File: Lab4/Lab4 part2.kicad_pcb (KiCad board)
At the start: 2 copper layers, 58.4 x 50.4 mm, 10 parts, among them J1 Conn_01x02_Male, U1 NE555D

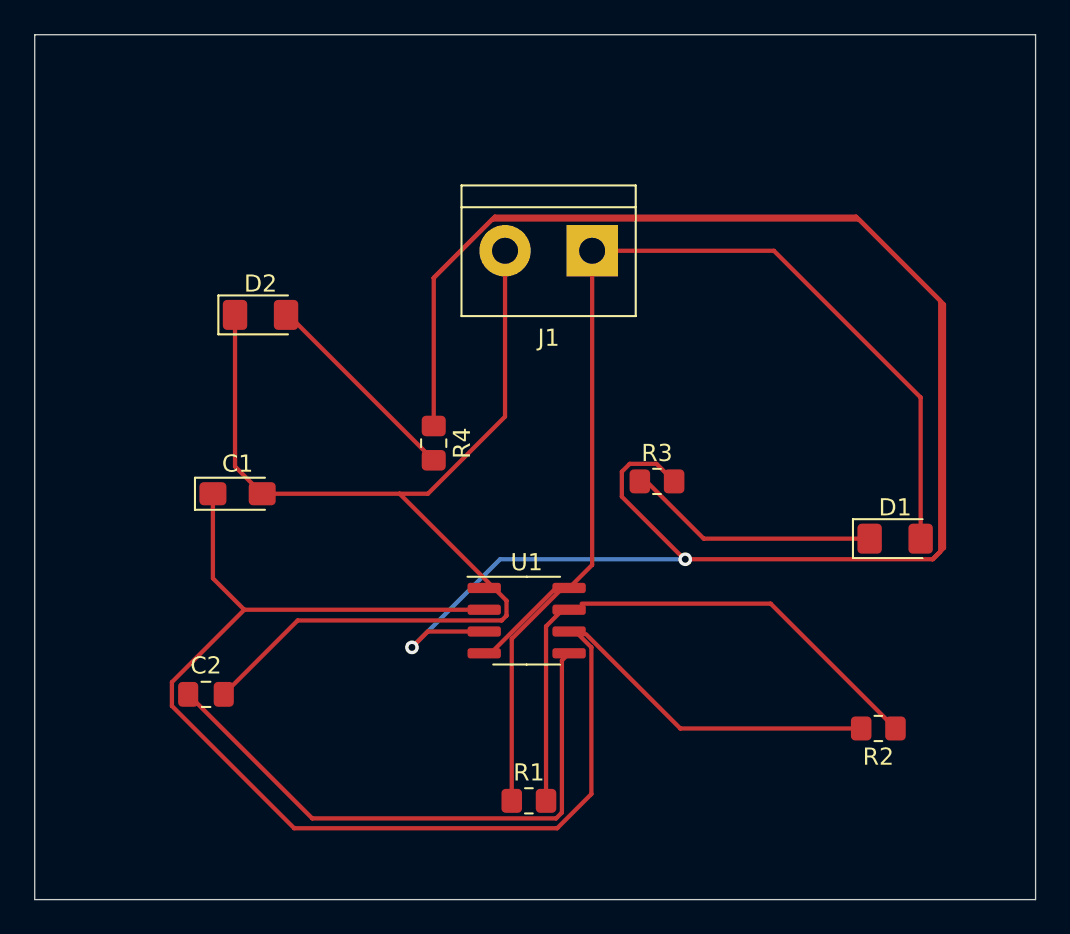
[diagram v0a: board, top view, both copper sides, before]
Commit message: update lab7
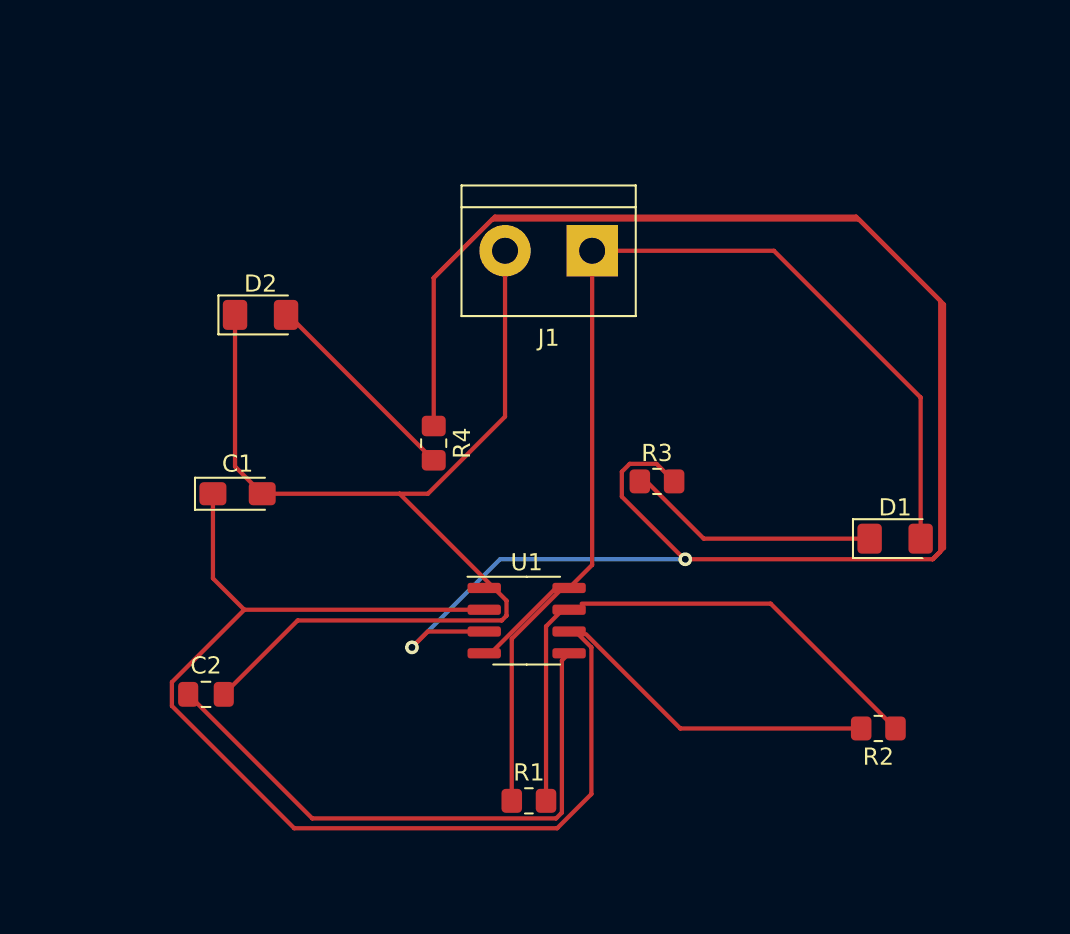
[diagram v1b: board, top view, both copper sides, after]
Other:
- board outline removed
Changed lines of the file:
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@@
       (outputformat 1)
       (mirror false)
-      (drillshape 0)
+      (drillshape 1)
       (scaleselection 1)
-      (outputdirectory "lab7/")
+      (outputdirectory "")
     )
   )
@@
     (fp_line (start 1.6 0.8) (end 1.6 -0.8) (layer "F.Fab") (width 0.1))
     (fp_line (start -1.2 -0.8) (end -1.6 -0.4) (layer "F.Fab") (width 0.1))
-    (pad "1" smd roundrect (at -1.4875 0) (size 1.425 1.75) (layers "F.Cu" "F.Paste" "F.Mask") (roundrect_rratio 0.1754392982)
+    (pad "1" smd roundrect (at -1.4875 0) (size 1.425 1.75) (layers "F.Cu" "F.Paste" "F.Mask") (roundrect_rratio 0.175439)
       (net 4 "Net-(D1-Pad1)") (pinfunction "K") (pintype "passive"))
-    (pad "2" smd roundrect (at 1.4875 0) (size 1.425 1.75) (layers "F.Cu" "F.Paste" "F.Mask") (roundrect_rratio 0.1754392982)
+    (pad "2" smd roundrect (at 1.4875 0) (size 1.425 1.75) (layers "F.Cu" "F.Paste" "F.Mask") (roundrect_rratio 0.175439)
       (net 5 "+9V") (pinfunction "A") (pintype "passive"))
     (model "${KICAD6_3DMODEL_DIR}/LED_SMD.3dshapes/LED_1206_3216Metric.wrl"
@@
     (fp_line (start 1.6 0.8) (end 1.6 -0.8) (layer "F.Fab") (width 0.1))
     (fp_line (start 1.6 -0.8) (end -1.2 -0.8) (layer "F.Fab") (width 0.1))
-    (pad "1" smd roundrect (at -1.4375 0) (size 1.575 1.35) (layers "F.Cu" "F.Paste" "F.Mask") (roundrect_rratio 0.1851851852)
+    (pad "1" smd roundrect (at -1.4375 0) (size 1.575 1.35) (layers "F.Cu" "F.Paste" "F.Mask") (roundrect_rratio 0.185185)
       (net 1 "/pin_2") (pintype "passive"))
-    (pad "2" smd roundrect (at 1.4375 0) (size 1.575 1.35) (layers "F.Cu" "F.Paste" "F.Mask") (roundrect_rratio 0.1851851852)
+    (pad "2" smd roundrect (at 1.4375 0) (size 1.575 1.35) (layers "F.Cu" "F.Paste" "F.Mask") (roundrect_rratio 0.185185)
       (net 2 "GND") (pintype "passive"))
     (model "${KICAD6_3DMODEL_DIR}/Capacitor_Tantalum_SMD.3dshapes/CP_EIA-3216-18_Kemet-A.wrl"
@@
     (fp_line (start -1 0.625) (end -1 -0.625) (layer "F.Fab") (width 0.1))
     (fp_line (start 1 -0.625) (end 1 0.625) (layer "F.Fab") (width 0.1))
-    (pad "1" smd roundrect (at -1 0 180) (size 1.2 1.4) (layers "F.Cu" "F.Paste" "F.Mask") (roundrect_rratio 0.2083333333)
+    (pad "1" smd roundrect (at -1 0 180) (size 1.2 1.4) (layers "F.Cu" "F.Paste" "F.Mask") (roundrect_rratio 0.208333)
       (net 7 "/pin_7") (pintype "passive"))
-    (pad "2" smd roundrect (at 1 0 180) (size 1.2 1.4) (layers "F.Cu" "F.Paste" "F.Mask") (roundrect_rratio 0.2083333333)
+    (pad "2" smd roundrect (at 1 0 180) (size 1.2 1.4) (layers "F.Cu" "F.Paste" "F.Mask") (roundrect_rratio 0.208333)
       (net 1 "/pin_2") (pintype "passive"))
     (model "${KICAD6_3DMODEL_DIR}/Resistor_SMD.3dshapes/R_0805_2012Metric.wrl"
@@
     (fp_line (start -1 0.625) (end -1 -0.625) (layer "F.Fab") (width 0.1))
     (fp_line (start -1 -0.625) (end 1 -0.625) (layer "F.Fab") (width 0.1))
-    (pad "1" smd roundrect (at -1 0) (size 1.2 1.4) (layers "F.Cu" "F.Paste" "F.Mask") (roundrect_rratio 0.2083333333)
+    (pad "1" smd roundrect (at -1 0) (size 1.2 1.4) (layers "F.Cu" "F.Paste" "F.Mask") (roundrect_rratio 0.208333)
       (net 5 "+9V") (pintype "passive"))
-    (pad "2" smd roundrect (at 1 0) (size 1.2 1.4) (layers "F.Cu" "F.Paste" "F.Mask") (roundrect_rratio 0.2083333333)
+    (pad "2" smd roundrect (at 1 0) (size 1.2 1.4) (layers "F.Cu" "F.Paste" "F.Mask") (roundrect_rratio 0.208333)
       (net 7 "/pin_7") (pintype "passive"))
     (model "${KICAD6_3DMODEL_DIR}/Resistor_SMD.3dshapes/R_0805_2012Metric.wrl"
@@
     (fp_line (start -1 0.625) (end -1 -0.625) (layer "F.Fab") (width 0.1))
     (fp_line (start 1 -0.625) (end 1 0.625) (layer "F.Fab") (width 0.1))
-    (pad "1" smd roundrect (at -1 0 270) (size 1.2 1.4) (layers "F.Cu" "F.Paste" "F.Mask") (roundrect_rratio 0.2083333333)
+    (pad "1" smd roundrect (at -1 0 270) (size 1.2 1.4) (layers "F.Cu" "F.Paste" "F.Mask") (roundrect_rratio 0.208333)
       (net 8 "/pin_3") (pintype "passive"))
-    (pad "2" smd roundrect (at 1 0 270) (size 1.2 1.4) (layers "F.Cu" "F.Paste" "F.Mask") (roundrect_rratio 0.2083333333)
+    (pad "2" smd roundrect (at 1 0 270) (size 1.2 1.4) (layers "F.Cu" "F.Paste" "F.Mask") (roundrect_rratio 0.208333)
       (net 6 "Net-(D2-Pad2)") (pintype "passive"))
     (model "${KICAD6_3DMODEL_DIR}/Resistor_SMD.3dshapes/R_0805_2012Metric.wrl"
@@
     (fp_line (start 1 0.625) (end -1 0.625) (layer "F.Fab") (width 0.1))
     (fp_line (start 1 -0.625) (end 1 0.625) (layer "F.Fab") (width 0.1))
-    (pad "1" smd roundrect (at -1.0375 0) (size 1.175 1.45) (layers "F.Cu" "F.Paste" "F.Mask") (roundrect_rratio 0.2127659574)
+    (pad "1" smd roundrect (at -1.0375 0) (size 1.175 1.45) (layers "F.Cu" "F.Paste" "F.Mask") (roundrect_rratio 0.212766)
       (net 3 "Net-(C2-Pad1)") (pintype "passive"))
-    (pad "2" smd roundrect (at 1.0375 0) (size 1.175 1.45) (layers "F.Cu" "F.Paste" "F.Mask") (roundrect_rratio 0.2127659574)
+    (pad "2" smd roundrect (at 1.0375 0) (size 1.175 1.45) (layers "F.Cu" "F.Paste" "F.Mask") (roundrect_rratio 0.212766)
       (net 2 "GND") (pintype "passive"))
     (model "${KICAD6_3DMODEL_DIR}/Capacitor_SMD.3dshapes/C_0805_2012Metric.wrl"
@@
     (fp_line (start 1 0.625) (end -1 0.625) (layer "F.Fab") (width 0.1))
     (fp_line (start 1 -0.625) (end 1 0.625) (layer "F.Fab") (width 0.1))
-    (pad "1" smd roundrect (at -1 0) (size 1.2 1.4) (layers "F.Cu" "F.Paste" "F.Mask") (roundrect_rratio 0.2083333333)
+    (pad "1" smd roundrect (at -1 0) (size 1.2 1.4) (layers "F.Cu" "F.Paste" "F.Mask") (roundrect_rratio 0.208333)
       (net 4 "Net-(D1-Pad1)") (pintype "passive"))
-    (pad "2" smd roundrect (at 1 0) (size 1.2 1.4) (layers "F.Cu" "F.Paste" "F.Mask") (roundrect_rratio 0.2083333333)
+    (pad "2" smd roundrect (at 1 0) (size 1.2 1.4) (layers "F.Cu" "F.Paste" "F.Mask") (roundrect_rratio 0.208333)
       (net 8 "/pin_3") (pintype "passive"))
     (model "${KICAD6_3DMODEL_DIR}/Resistor_SMD.3dshapes/R_0805_2012Metric.wrl"
@@
     (fp_line (start 1.6 -0.8) (end -1.2 -0.8) (layer "F.Fab") (width 0.1))
     (fp_line (start -1.2 -0.8) (end -1.6 -0.4) (layer "F.Fab") (width 0.1))
-    (pad "1" smd roundrect (at -1.4875 0) (size 1.425 1.75) (layers "F.Cu" "F.Paste" "F.Mask") (roundrect_rratio 0.1754392982)
+    (pad "1" smd roundrect (at -1.4875 0) (size 1.425 1.75) (layers "F.Cu" "F.Paste" "F.Mask") (roundrect_rratio 0.175439)
       (net 2 "GND") (pinfunction "K") (pintype "passive"))
-    (pad "2" smd roundrect (at 1.4875 0) (size 1.425 1.75) (layers "F.Cu" "F.Paste" "F.Mask") (roundrect_rratio 0.1754392982)
+    (pad "2" smd roundrect (at 1.4875 0) (size 1.425 1.75) (layers "F.Cu" "F.Paste" "F.Mask") (roundrect_rratio 0.175439)
       (net 6 "Net-(D2-Pad2)") (pinfunction "A") (pintype "passive"))
     (model "${KICAD6_3DMODEL_DIR}/LED_SMD.3dshapes/LED_1206_3216Metric.wrl"
@@
     )
   )
-  (gr_rect (start 110.83 57.61) (end 169.2 108.05) (layer "Edge.Cuts") (width 0.05) (fill none))
   (segment (start 121.2225 84.38) (end 121.2225 89.3125) (width 0.25) (layer "F.Cu") (net 1))
   (segment (start 123.055 91.145) (end 137.045 91.145) (width 0.25) (layer "F.Cu") (net 1))

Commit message: my lab8 update, tks
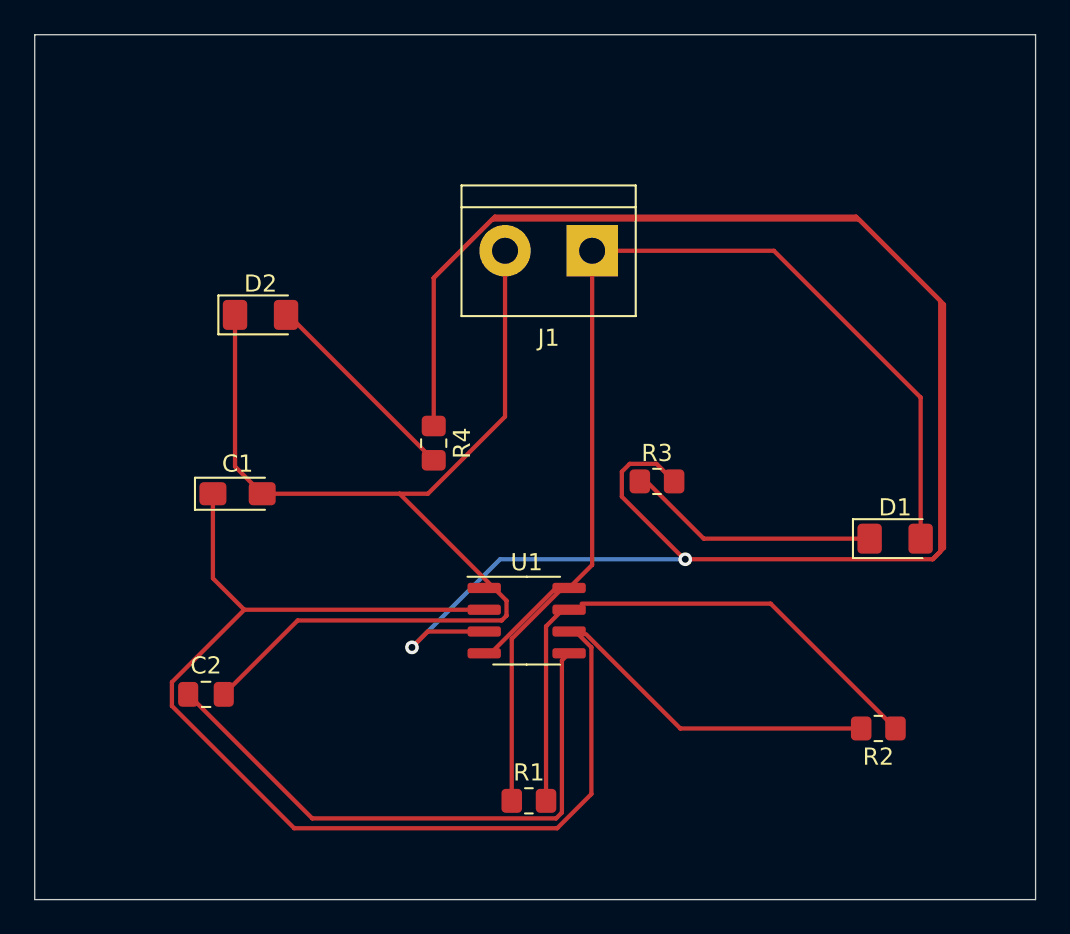
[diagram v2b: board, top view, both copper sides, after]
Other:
- board outline added: 58.4 x 50.4 mm
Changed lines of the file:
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@@
       (outputformat 1)
       (mirror false)
-      (drillshape 1)
+      (drillshape 0)
       (scaleselection 1)
-      (outputdirectory "")
+      (outputdirectory "lab7/")
     )
   )
@@
     (fp_line (start 1.6 0.8) (end 1.6 -0.8) (layer "F.Fab") (width 0.1))
     (fp_line (start -1.2 -0.8) (end -1.6 -0.4) (layer "F.Fab") (width 0.1))
-    (pad "1" smd roundrect (at -1.4875 0) (size 1.425 1.75) (layers "F.Cu" "F.Paste" "F.Mask") (roundrect_rratio 0.175439)
+    (pad "1" smd roundrect (at -1.4875 0) (size 1.425 1.75) (layers "F.Cu" "F.Paste" "F.Mask") (roundrect_rratio 0.1754392982)
       (net 4 "Net-(D1-Pad1)") (pinfunction "K") (pintype "passive"))
-    (pad "2" smd roundrect (at 1.4875 0) (size 1.425 1.75) (layers "F.Cu" "F.Paste" "F.Mask") (roundrect_rratio 0.175439)
+    (pad "2" smd roundrect (at 1.4875 0) (size 1.425 1.75) (layers "F.Cu" "F.Paste" "F.Mask") (roundrect_rratio 0.1754392982)
       (net 5 "+9V") (pinfunction "A") (pintype "passive"))
     (model "${KICAD6_3DMODEL_DIR}/LED_SMD.3dshapes/LED_1206_3216Metric.wrl"
@@
     (fp_line (start 1.6 0.8) (end 1.6 -0.8) (layer "F.Fab") (width 0.1))
     (fp_line (start 1.6 -0.8) (end -1.2 -0.8) (layer "F.Fab") (width 0.1))
-    (pad "1" smd roundrect (at -1.4375 0) (size 1.575 1.35) (layers "F.Cu" "F.Paste" "F.Mask") (roundrect_rratio 0.185185)
+    (pad "1" smd roundrect (at -1.4375 0) (size 1.575 1.35) (layers "F.Cu" "F.Paste" "F.Mask") (roundrect_rratio 0.1851851852)
       (net 1 "/pin_2") (pintype "passive"))
-    (pad "2" smd roundrect (at 1.4375 0) (size 1.575 1.35) (layers "F.Cu" "F.Paste" "F.Mask") (roundrect_rratio 0.185185)
+    (pad "2" smd roundrect (at 1.4375 0) (size 1.575 1.35) (layers "F.Cu" "F.Paste" "F.Mask") (roundrect_rratio 0.1851851852)
       (net 2 "GND") (pintype "passive"))
     (model "${KICAD6_3DMODEL_DIR}/Capacitor_Tantalum_SMD.3dshapes/CP_EIA-3216-18_Kemet-A.wrl"
@@
     (fp_line (start -1 0.625) (end -1 -0.625) (layer "F.Fab") (width 0.1))
     (fp_line (start 1 -0.625) (end 1 0.625) (layer "F.Fab") (width 0.1))
-    (pad "1" smd roundrect (at -1 0 180) (size 1.2 1.4) (layers "F.Cu" "F.Paste" "F.Mask") (roundrect_rratio 0.208333)
+    (pad "1" smd roundrect (at -1 0 180) (size 1.2 1.4) (layers "F.Cu" "F.Paste" "F.Mask") (roundrect_rratio 0.2083333333)
       (net 7 "/pin_7") (pintype "passive"))
-    (pad "2" smd roundrect (at 1 0 180) (size 1.2 1.4) (layers "F.Cu" "F.Paste" "F.Mask") (roundrect_rratio 0.208333)
+    (pad "2" smd roundrect (at 1 0 180) (size 1.2 1.4) (layers "F.Cu" "F.Paste" "F.Mask") (roundrect_rratio 0.2083333333)
       (net 1 "/pin_2") (pintype "passive"))
     (model "${KICAD6_3DMODEL_DIR}/Resistor_SMD.3dshapes/R_0805_2012Metric.wrl"
@@
     (fp_line (start -1 0.625) (end -1 -0.625) (layer "F.Fab") (width 0.1))
     (fp_line (start -1 -0.625) (end 1 -0.625) (layer "F.Fab") (width 0.1))
-    (pad "1" smd roundrect (at -1 0) (size 1.2 1.4) (layers "F.Cu" "F.Paste" "F.Mask") (roundrect_rratio 0.208333)
+    (pad "1" smd roundrect (at -1 0) (size 1.2 1.4) (layers "F.Cu" "F.Paste" "F.Mask") (roundrect_rratio 0.2083333333)
       (net 5 "+9V") (pintype "passive"))
-    (pad "2" smd roundrect (at 1 0) (size 1.2 1.4) (layers "F.Cu" "F.Paste" "F.Mask") (roundrect_rratio 0.208333)
+    (pad "2" smd roundrect (at 1 0) (size 1.2 1.4) (layers "F.Cu" "F.Paste" "F.Mask") (roundrect_rratio 0.2083333333)
       (net 7 "/pin_7") (pintype "passive"))
     (model "${KICAD6_3DMODEL_DIR}/Resistor_SMD.3dshapes/R_0805_2012Metric.wrl"
@@
     (fp_line (start -1 0.625) (end -1 -0.625) (layer "F.Fab") (width 0.1))
     (fp_line (start 1 -0.625) (end 1 0.625) (layer "F.Fab") (width 0.1))
-    (pad "1" smd roundrect (at -1 0 270) (size 1.2 1.4) (layers "F.Cu" "F.Paste" "F.Mask") (roundrect_rratio 0.208333)
+    (pad "1" smd roundrect (at -1 0 270) (size 1.2 1.4) (layers "F.Cu" "F.Paste" "F.Mask") (roundrect_rratio 0.2083333333)
       (net 8 "/pin_3") (pintype "passive"))
-    (pad "2" smd roundrect (at 1 0 270) (size 1.2 1.4) (layers "F.Cu" "F.Paste" "F.Mask") (roundrect_rratio 0.208333)
+    (pad "2" smd roundrect (at 1 0 270) (size 1.2 1.4) (layers "F.Cu" "F.Paste" "F.Mask") (roundrect_rratio 0.2083333333)
       (net 6 "Net-(D2-Pad2)") (pintype "passive"))
     (model "${KICAD6_3DMODEL_DIR}/Resistor_SMD.3dshapes/R_0805_2012Metric.wrl"
@@
     (fp_line (start 1 0.625) (end -1 0.625) (layer "F.Fab") (width 0.1))
     (fp_line (start 1 -0.625) (end 1 0.625) (layer "F.Fab") (width 0.1))
-    (pad "1" smd roundrect (at -1.0375 0) (size 1.175 1.45) (layers "F.Cu" "F.Paste" "F.Mask") (roundrect_rratio 0.212766)
+    (pad "1" smd roundrect (at -1.0375 0) (size 1.175 1.45) (layers "F.Cu" "F.Paste" "F.Mask") (roundrect_rratio 0.2127659574)
       (net 3 "Net-(C2-Pad1)") (pintype "passive"))
-    (pad "2" smd roundrect (at 1.0375 0) (size 1.175 1.45) (layers "F.Cu" "F.Paste" "F.Mask") (roundrect_rratio 0.212766)
+    (pad "2" smd roundrect (at 1.0375 0) (size 1.175 1.45) (layers "F.Cu" "F.Paste" "F.Mask") (roundrect_rratio 0.2127659574)
       (net 2 "GND") (pintype "passive"))
     (model "${KICAD6_3DMODEL_DIR}/Capacitor_SMD.3dshapes/C_0805_2012Metric.wrl"
@@
     (fp_line (start 1 0.625) (end -1 0.625) (layer "F.Fab") (width 0.1))
     (fp_line (start 1 -0.625) (end 1 0.625) (layer "F.Fab") (width 0.1))
-    (pad "1" smd roundrect (at -1 0) (size 1.2 1.4) (layers "F.Cu" "F.Paste" "F.Mask") (roundrect_rratio 0.208333)
+    (pad "1" smd roundrect (at -1 0) (size 1.2 1.4) (layers "F.Cu" "F.Paste" "F.Mask") (roundrect_rratio 0.2083333333)
       (net 4 "Net-(D1-Pad1)") (pintype "passive"))
-    (pad "2" smd roundrect (at 1 0) (size 1.2 1.4) (layers "F.Cu" "F.Paste" "F.Mask") (roundrect_rratio 0.208333)
+    (pad "2" smd roundrect (at 1 0) (size 1.2 1.4) (layers "F.Cu" "F.Paste" "F.Mask") (roundrect_rratio 0.2083333333)
       (net 8 "/pin_3") (pintype "passive"))
     (model "${KICAD6_3DMODEL_DIR}/Resistor_SMD.3dshapes/R_0805_2012Metric.wrl"
@@
     (fp_line (start 1.6 -0.8) (end -1.2 -0.8) (layer "F.Fab") (width 0.1))
     (fp_line (start -1.2 -0.8) (end -1.6 -0.4) (layer "F.Fab") (width 0.1))
-    (pad "1" smd roundrect (at -1.4875 0) (size 1.425 1.75) (layers "F.Cu" "F.Paste" "F.Mask") (roundrect_rratio 0.175439)
+    (pad "1" smd roundrect (at -1.4875 0) (size 1.425 1.75) (layers "F.Cu" "F.Paste" "F.Mask") (roundrect_rratio 0.1754392982)
       (net 2 "GND") (pinfunction "K") (pintype "passive"))
-    (pad "2" smd roundrect (at 1.4875 0) (size 1.425 1.75) (layers "F.Cu" "F.Paste" "F.Mask") (roundrect_rratio 0.175439)
+    (pad "2" smd roundrect (at 1.4875 0) (size 1.425 1.75) (layers "F.Cu" "F.Paste" "F.Mask") (roundrect_rratio 0.1754392982)
       (net 6 "Net-(D2-Pad2)") (pinfunction "A") (pintype "passive"))
     (model "${KICAD6_3DMODEL_DIR}/LED_SMD.3dshapes/LED_1206_3216Metric.wrl"
@@
     )
   )
+  (gr_rect (start 110.83 57.61) (end 169.2 108.05) (layer "Edge.Cuts") (width 0.05) (fill none))
   (segment (start 121.2225 84.38) (end 121.2225 89.3125) (width 0.25) (layer "F.Cu") (net 1))
   (segment (start 123.055 91.145) (end 137.045 91.145) (width 0.25) (layer "F.Cu") (net 1))
